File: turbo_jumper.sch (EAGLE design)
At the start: 21 parts, among them J1 10090926-P264XLF, K1 G6K-2P-Y, K2 G6K-2P-Y, X1 E74

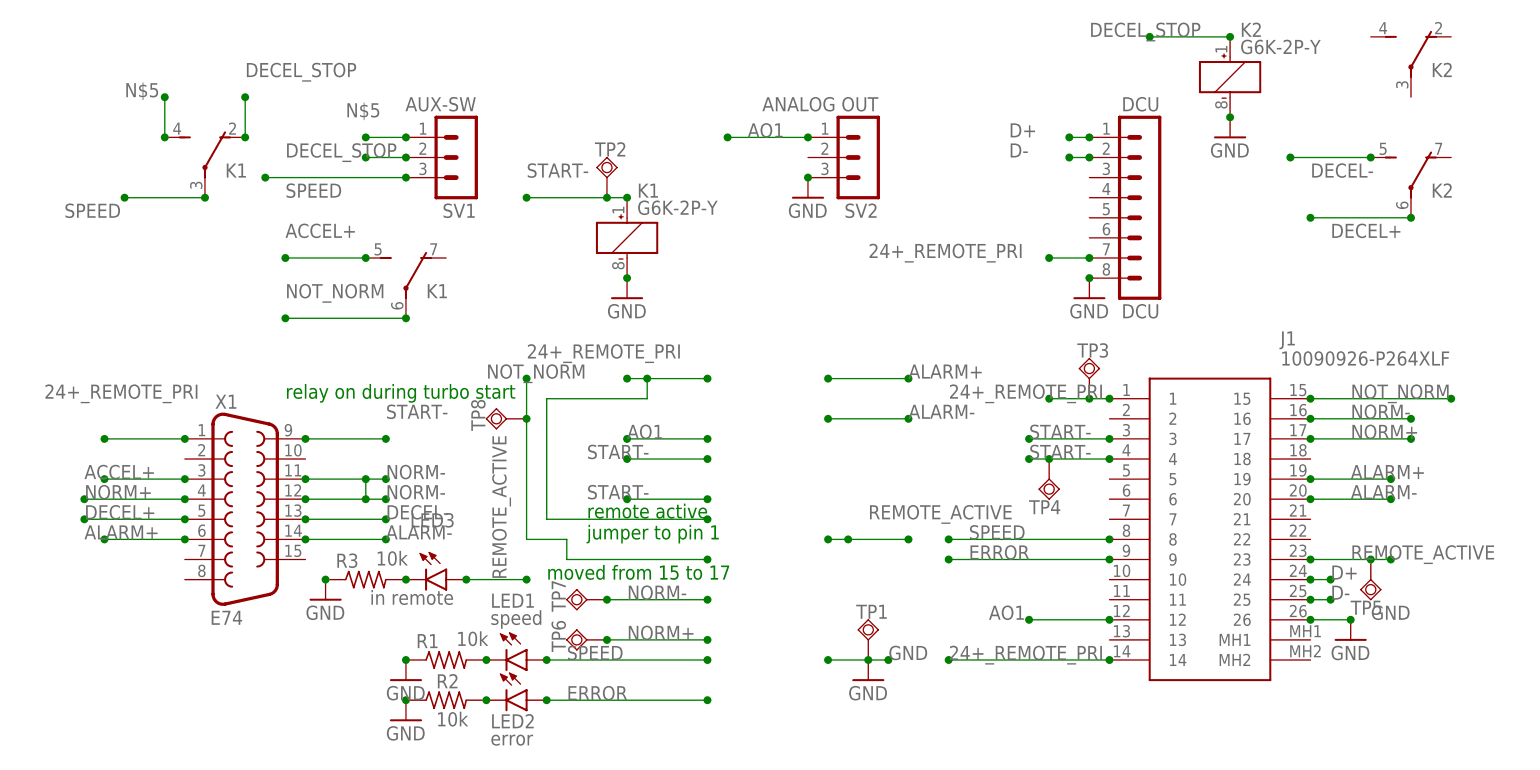
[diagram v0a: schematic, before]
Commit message: up
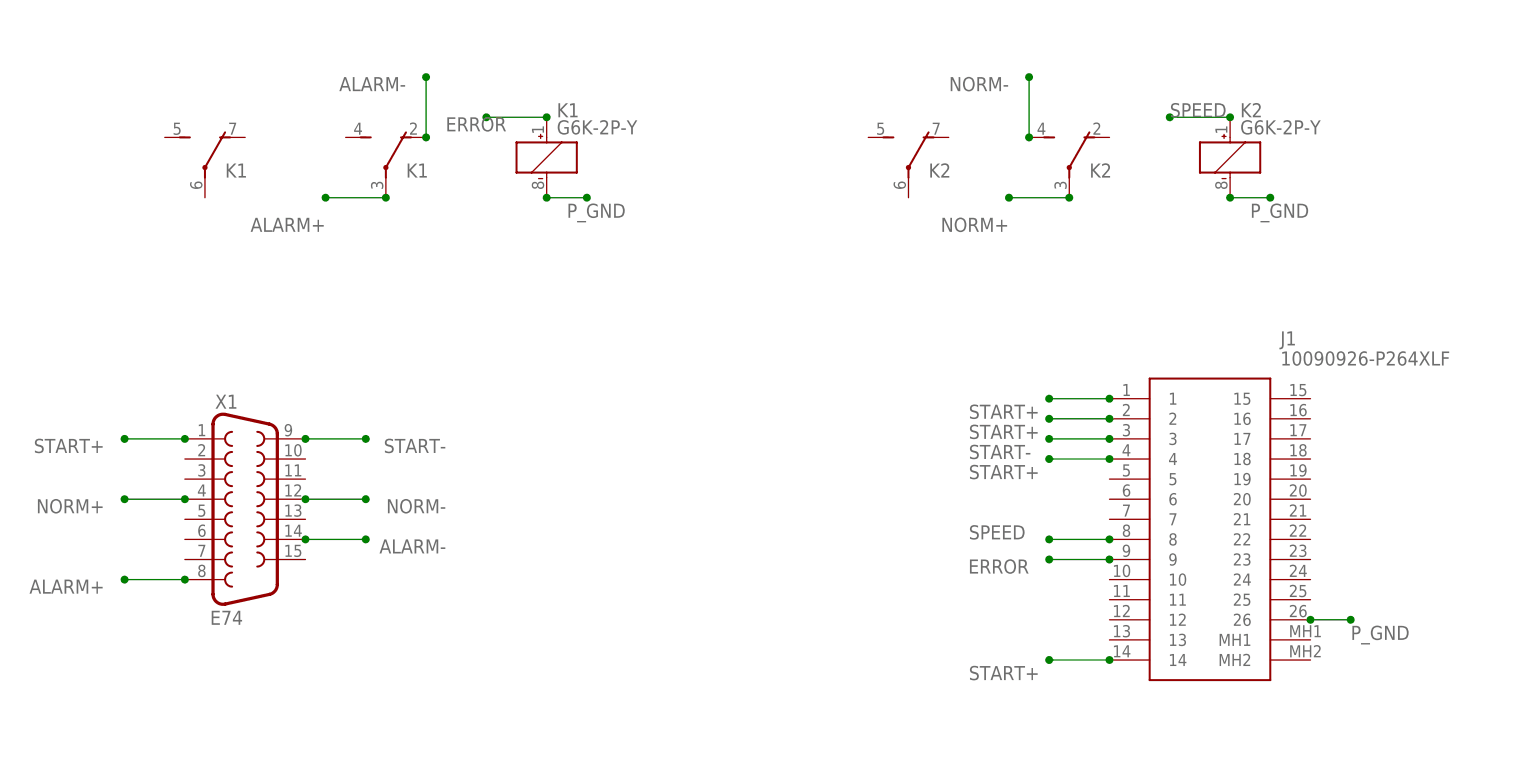
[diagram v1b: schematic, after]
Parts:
- removed DCU: DCU, con-lstb:MA08-1
- removed LED1: speed, led:LEDCHIPLED_1206
- removed LED2: error, led:LEDCHIPLED_1206
- removed LED3: in remote, led:LEDCHIPLED_1206
- removed R1, R2, R3: 10k, rcl:R-US_M1206
- removed SV1: AUX-SW, con-lstb:MA03-1
- removed SV2: ANALOG OUT, con-lstb:MA03-1
- removed TP1, TP2, TP3, TP4, TP5, TP6, TP7, TP8: TPSQTP13R, testpad:TPSQTP13R
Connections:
- removed net 24+_REMOTE_PRI: DCU.7, J1.1, J1.14, TP3.TP, X1.1
- removed net ACCEL+: K13.S, X1.3
- removed net AO1: J1.12, SV2.1
- removed net D+: DCU.1, J1.24
- removed net D-: DCU.2, J1.25
- removed net DECEL+: K23.P, X1.5
- removed net DECEL-: K23.S, X1.13
- removed net DECEL_STOP: K12.O, K21.+, SV1.2
- removed net GND: DCU.8, J1.26, K11.-, K21.-, R1.1, R2.1, R3.1, SV2.3, TP1.TP
- removed net N$2: LED3.C, R3.2
- removed net N$3: LED1.C, R1.2
- removed net N$4: LED2.C, R2.2
- removed net N$5: K12.S, SV1.1
- removed net NOT_NORM: J1.15, K13.P, TP8.TP
- removed net REMOTE_ACTIVE: J1.23, LED3.A, TP5.TP
- new net P_GND: J1.26, K11.-, K21.-
- new net START+: J1.1, J1.14, J1.2, J1.4, X1.1
- net ALARM+: now also K12.P, X1.8; no longer J1.19, X1.6
- net ALARM-: now also K12.O; no longer J1.20
- net ERROR: now also K11.+; no longer LED2.A
- net NORM+: now also K22.P; no longer J1.17, TP6.TP
- net NORM-: now also K22.S; no longer J1.16, TP7.TP, X1.11
- net SPEED: now also K21.+; no longer K12.P, LED1.A, SV1.3
- net START-: no longer J1.4, K11.+, TP2.TP, TP4.TP
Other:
- note removed: "moved from 15 to 17"
- note removed: "relay on during turbo start"
- note removed: "remote active jumper to pin 1"
- moved on the sheet: K1, K2
